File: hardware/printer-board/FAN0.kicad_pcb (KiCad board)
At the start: 2 copper layers, 8 parts, among them J38 TO FAN1, Q4 D882

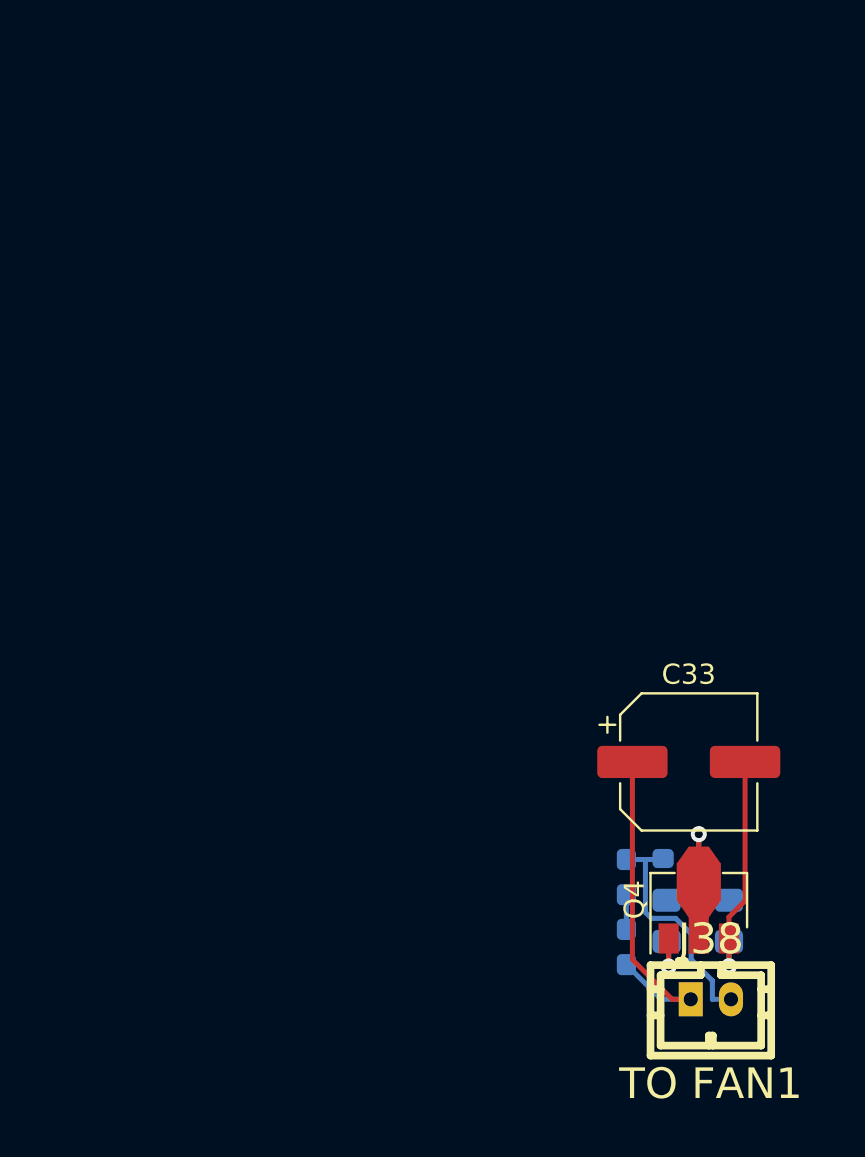
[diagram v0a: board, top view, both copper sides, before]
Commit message: update,
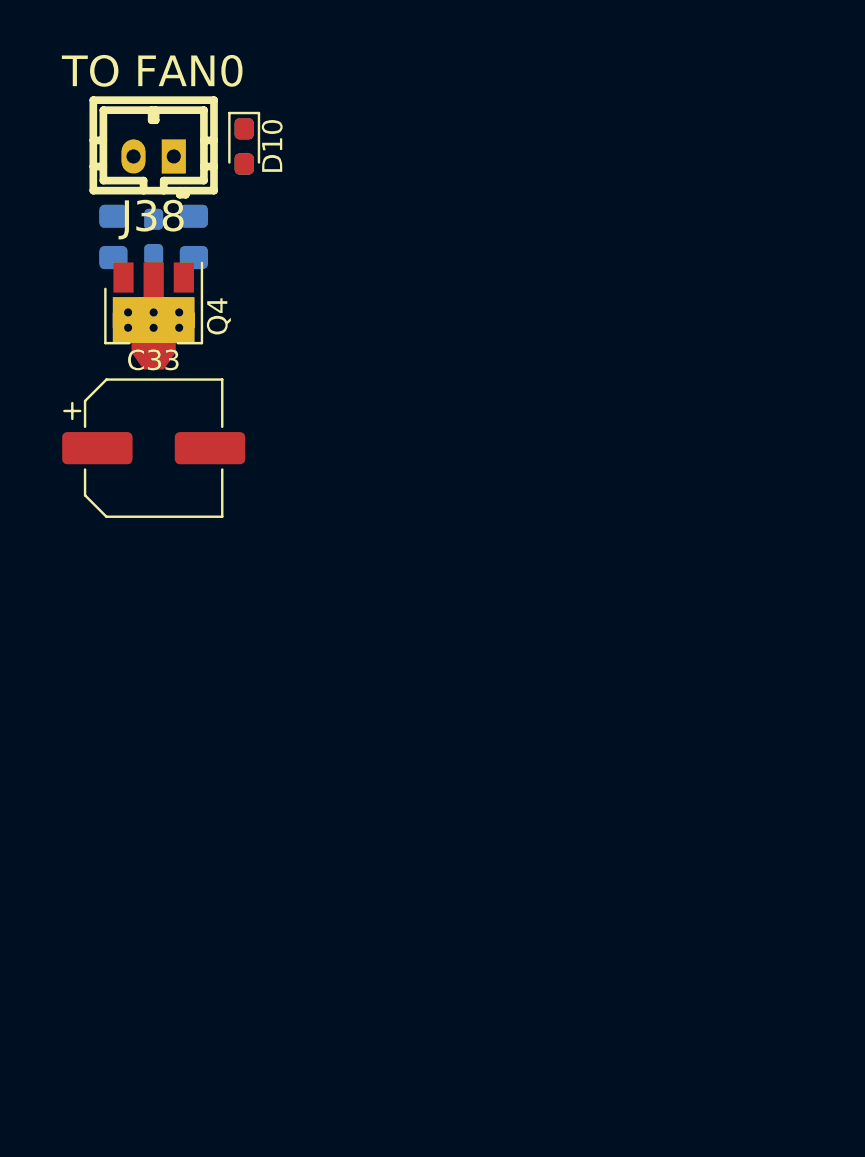
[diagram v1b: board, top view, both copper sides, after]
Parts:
- D10: moved to F.Cu
- J38: value TO FAN1 -> TO FAN0
- Q4: footprint Package_TO_SOT_SMD:SOT-89-3 -> footprint-lib:SOT-89-3,thermal_vias
- moved J38 50.2 mm to (6.00, 5.00), turned to 180 degrees
- moved R44 45.7 mm to (4.00, 9.00)
- moved R43 42.4 mm to (6.00, 9.00), turned to 90 degrees
- moved R36 41.5 mm to (10.5, 4.50), turned to 270 degrees
- moved R42 41.3 mm to (8.00, 9.00)
- moved D10 41.0 mm to (10.5, 4.50)
- moved Q4 40.4 mm to (6.00, 12.5), turned to 270 degrees
- moved C33 30.8 mm to (6.00, 19.5)
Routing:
- net +12V: track 17.5 -> 0.00 mm
- net Net-(D10-Pad1): track 11.8 -> 0.00 mm
- net GND: track 11.7 -> 0.00 mm, vias 1 -> 0
- net Net-(Q4-Pad2): track 6.27 -> 0.00 mm, vias 1 -> 0
- net /FAN_EN: track 3.10 -> 0.00 mm
- net Net-(Q4-Pad1): track 2.67 -> 0.00 mm, vias 1 -> 0
- net Net-(D10-Pad2): track 1.72 -> 0.00 mm
